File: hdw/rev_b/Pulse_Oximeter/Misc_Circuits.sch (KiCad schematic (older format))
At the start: 9 parts, among them J2001 I2C, J2002 USB UART, U2001 MCP9804

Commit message: changed all passives to 0402, cleared digikey pns
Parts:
- C2001: Digi-Key PN 490-10701-1-ND -> (none)
- R2001, R?: Digi-Key PN RMCF0402FT10K0CT-ND -> (none)
- R2002, R?: Digi-Key PN 541-3964-1-ND -> (none)
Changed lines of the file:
@@
 F 5 "1%" H 5670 4930 50  0000 L CNN "Tolerance"
 F 6 "1/16W" H 5680 4850 50  0000 L CNN "Wattage"
-F 7 "RMCF0402FT10K0CT-ND" H 5570 4930 50  0001 C CNN "Digi-Key PN"
+F 7 "" H 5570 4930 50  0001 C CNN "Digi-Key PN"
 	1    5570 4930
 	1    0    0    -1
@@
 F 6 "1/16W" H 5680 5310 50  0000 L CNN "Wattage"
 F 7 "Telemetry" H 5680 5230 50  0000 L CNN "Configuration"
-F 8 "541-3964-1-ND" H 5570 5390 50  0001 C CNN "Digi-Key PN"
+F 8 "" H 5570 5390 50  0001 C CNN "Digi-Key PN"
 	1    5570 5390
 	1    0    0    -1
@@
 F 5 "50V" H 5050 3390 50  0000 R CNN "Voltage"
 F 6 "X7R" H 5050 3290 50  0000 R CNN "Dielectric"
-F 7 "490-10701-1-ND" H 1290 -3490 50  0001 C CNN "Digi-Key PN"
+F 7 "" H 1290 -3490 50  0001 C CNN "Digi-Key PN"
 F 8 "Telemetry" H 4670 3390 50  0000 C CNN "Configuration"
 	1    5200 3390
@@
 F 5 "1%" H 6870 4930 50  0000 L CNN "Tolerance"
 F 6 "1/16W" H 6880 4850 50  0000 L CNN "Wattage"
-F 7 "RMCF0402FT10K0CT-ND" H 6770 4930 50  0001 C CNN "Digi-Key PN"
+F 7 "" H 6770 4930 50  0001 C CNN "Digi-Key PN"
 	1    6770 4930
 	1    0    0    -1
@@
 F 6 "1/16W" H 6880 5310 50  0000 L CNN "Wattage"
 F 7 "ETC" H 6880 5230 50  0000 L CNN "Configuration"
-F 8 "541-3964-1-ND" H 6770 5390 50  0001 C CNN "Digi-Key PN"
+F 8 "" H 6770 5390 50  0001 C CNN "Digi-Key PN"
 	1    6770 5390
 	1    0    0    -1

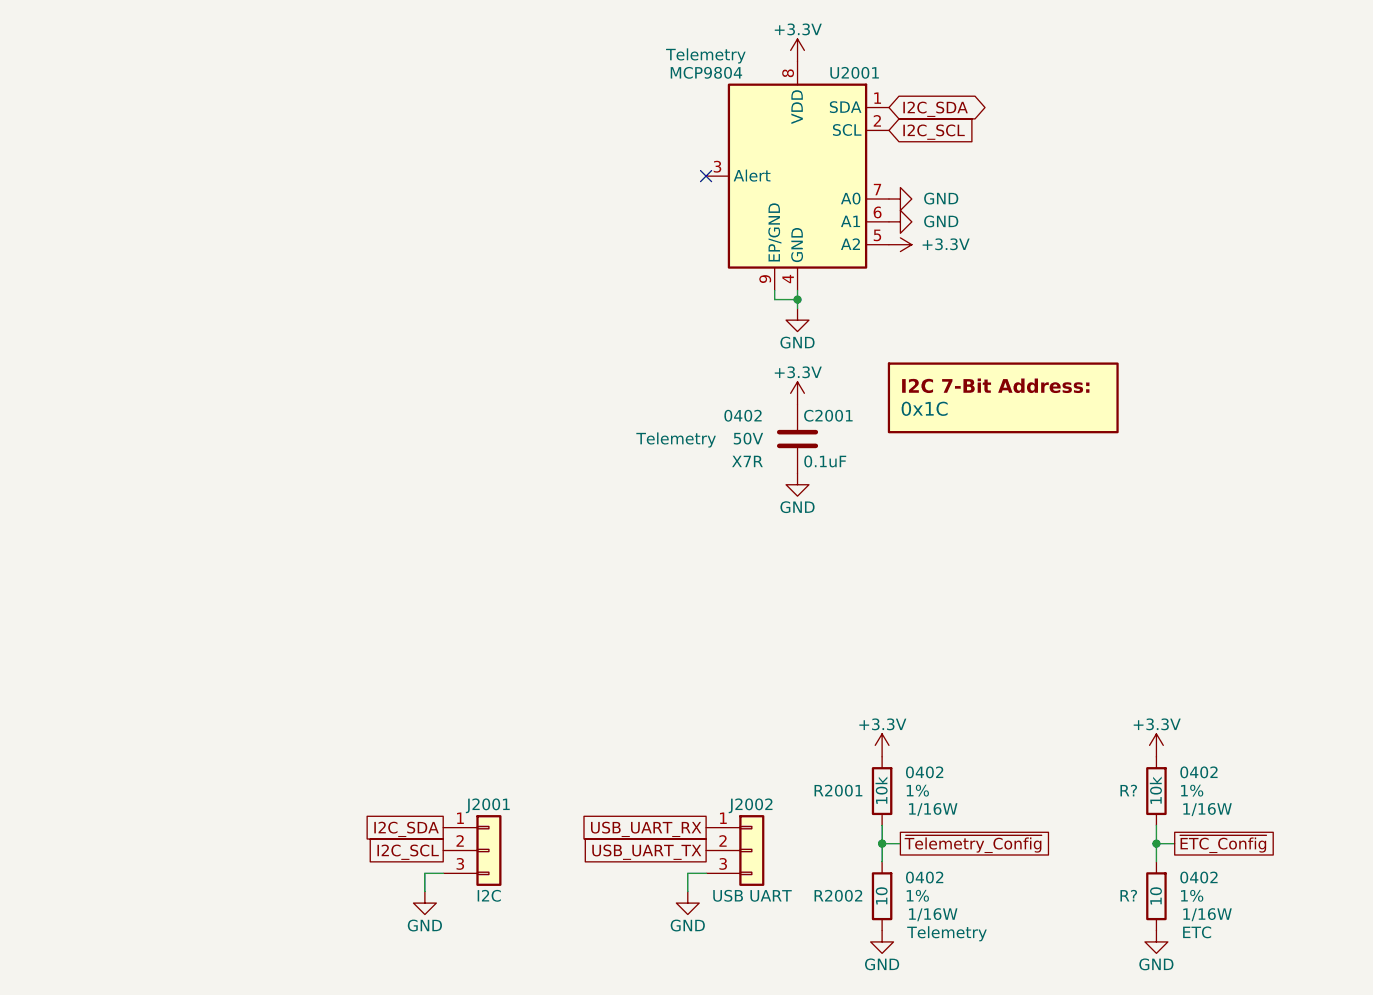
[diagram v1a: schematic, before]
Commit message: few little tweaks
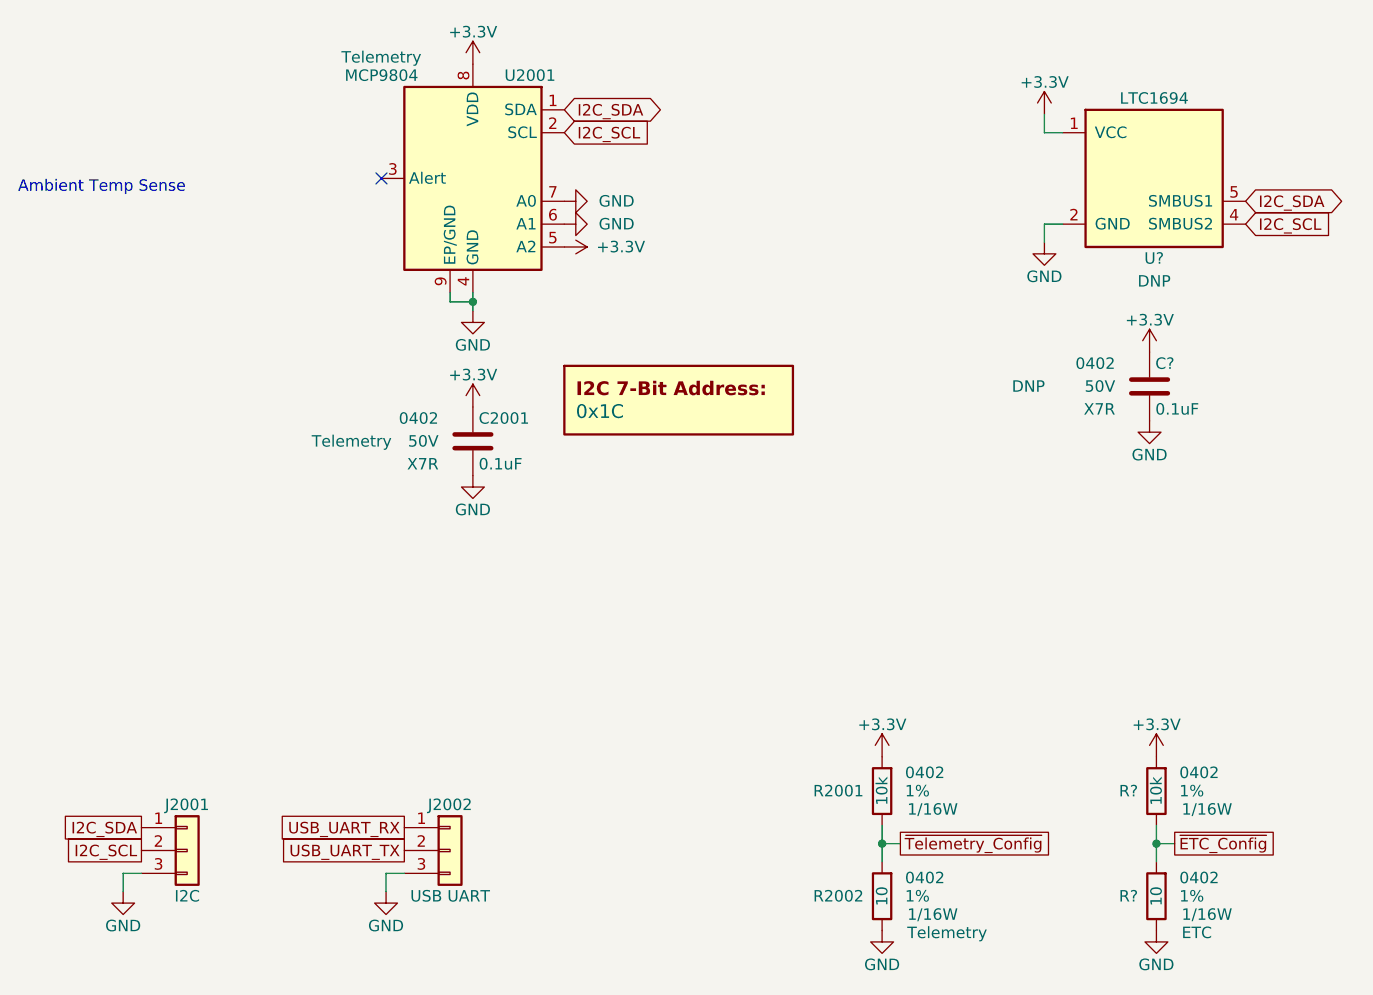
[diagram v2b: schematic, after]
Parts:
- added C?: 0.1uF, Capacitors_SMD:C_0402, symbol Custom_Library:C_Custom
- added U?: LTC1694, Package_TO_SOT_SMD:SOT-23-5, symbol Custom_Library:LTC1694
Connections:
- net +3V3: now also C?.1, U?.1 (VCC)
- net GND: now also C?.2, U?.2 (GND)
- net I2C_SCL: now also U?.4 (SMBUS2)
- net I2C_SDA: now also U?.5 (SMBUS1)
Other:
- note added: "Ambient Temp Sense"
- moved on the sheet: C2001, J2001, J2002, U2001
